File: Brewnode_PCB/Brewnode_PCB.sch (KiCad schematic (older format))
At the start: 6 parts

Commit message: Done PCB Sch Work
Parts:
- R1, R2: footprint (none) -> Resistor_SMD:R_0805_2012Metric_Pad1.15x1.40mm_HandSolder
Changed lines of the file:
@@
 F 0 "R1" V 2193 1100 50  0000 C CNN
 F 1 "220Ohm" V 2284 1100 50  0000 C CNN
-F 2 "" V 2330 1100 50  0001 C CNN
+F 2 "Resistor_SMD:R_0805_2012Metric_Pad1.15x1.40mm_HandSolder" V 2330 1100 50  0001 C CNN
 F 3 "https://datasheet.lcsc.com/szlcsc/1810241809_UNI-ROYAL-Uniroyal-Elec-0805W8F2200T5E_C17557.pdf" H 2400 1100 50  0001 C CNN
 F 4 "C17557" H 2400 1100 50  0001 C CNN "LCSC"
@@
 F 0 "R2" V 2193 1500 50  0000 C CNN
 F 1 "100Ohm" V 2284 1500 50  0000 C CNN
-F 2 "" V 2330 1500 50  0001 C CNN
+F 2 "Resistor_SMD:R_0805_2012Metric_Pad1.15x1.40mm_HandSolder" V 2330 1500 50  0001 C CNN
 F 3 "https://datasheet.lcsc.com/szlcsc/1809062111_UNI-ROYAL-Uniroyal-Elec-0805W8F1000T5E_C17408.pdf" H 2400 1500 50  0001 C CNN
 F 4 "C17408" H 2400 1500 50  0001 C CNN "LCSC"

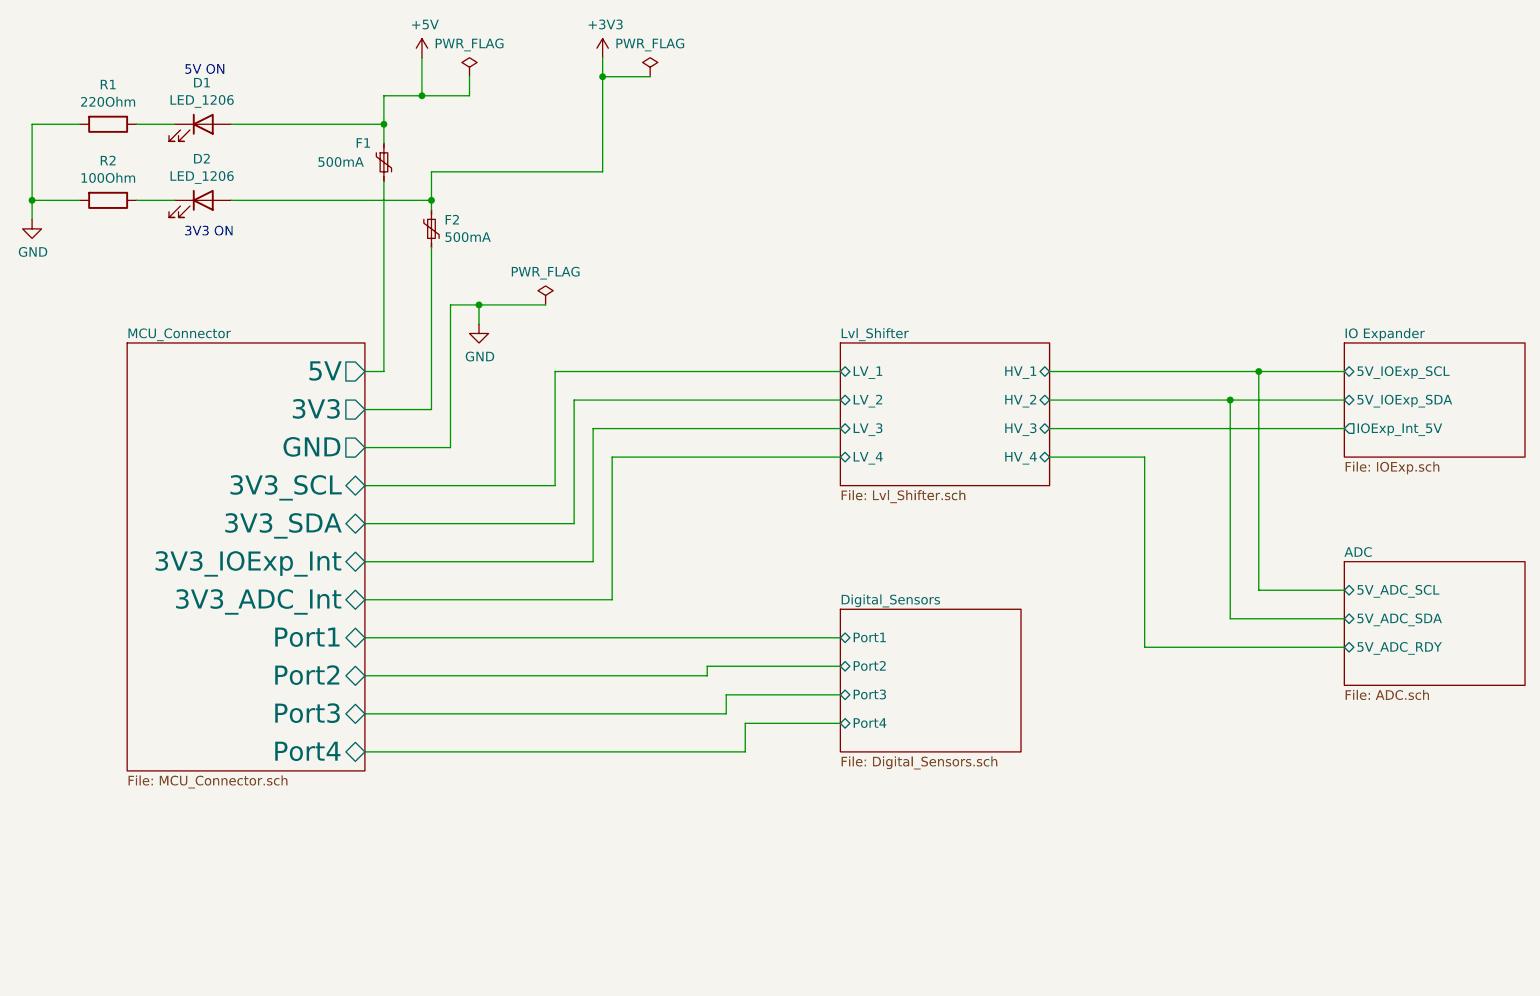
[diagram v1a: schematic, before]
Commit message: More PCB Pcb work
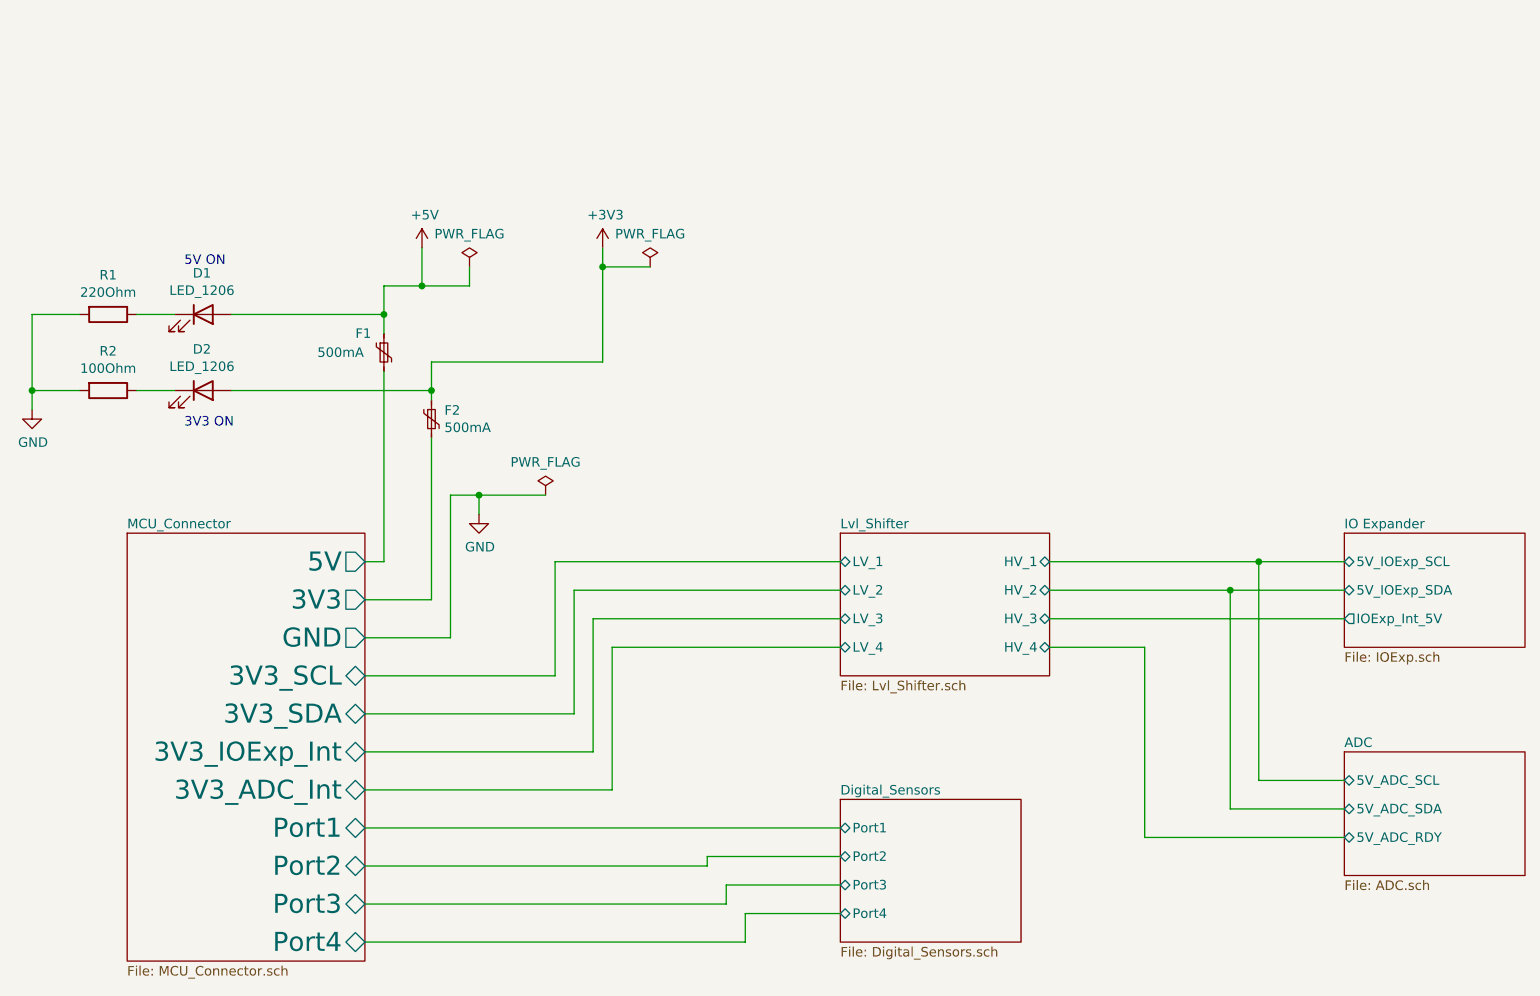
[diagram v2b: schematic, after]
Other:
- moved on the sheet: D1, D2, F1, F2, R1, R2
